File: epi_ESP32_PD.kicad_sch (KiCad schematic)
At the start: 53 parts, among them J1 Conn_01x08, J2 USB_C_Receptacle_USB2.0, J3 Conn_01x08, J4 Conn_01x02, J5 Conn_01x06, Q1 Q_PMOS_GDS, Q2 Q_NMOS_GDS, Q3 Q_NMOS_GDS, Q4 Q_NMOS_GDS, Q5 Q_NMOS_GDS, Q6 Q_NMOS_GDS, SW1 SW_MEC_5G, SW2 SW_MEC_5G, U1 ESP32-C3, U2 MIC5219-5.0YM5, U4 MIC5219-3.3YM5, Y1 Crystal

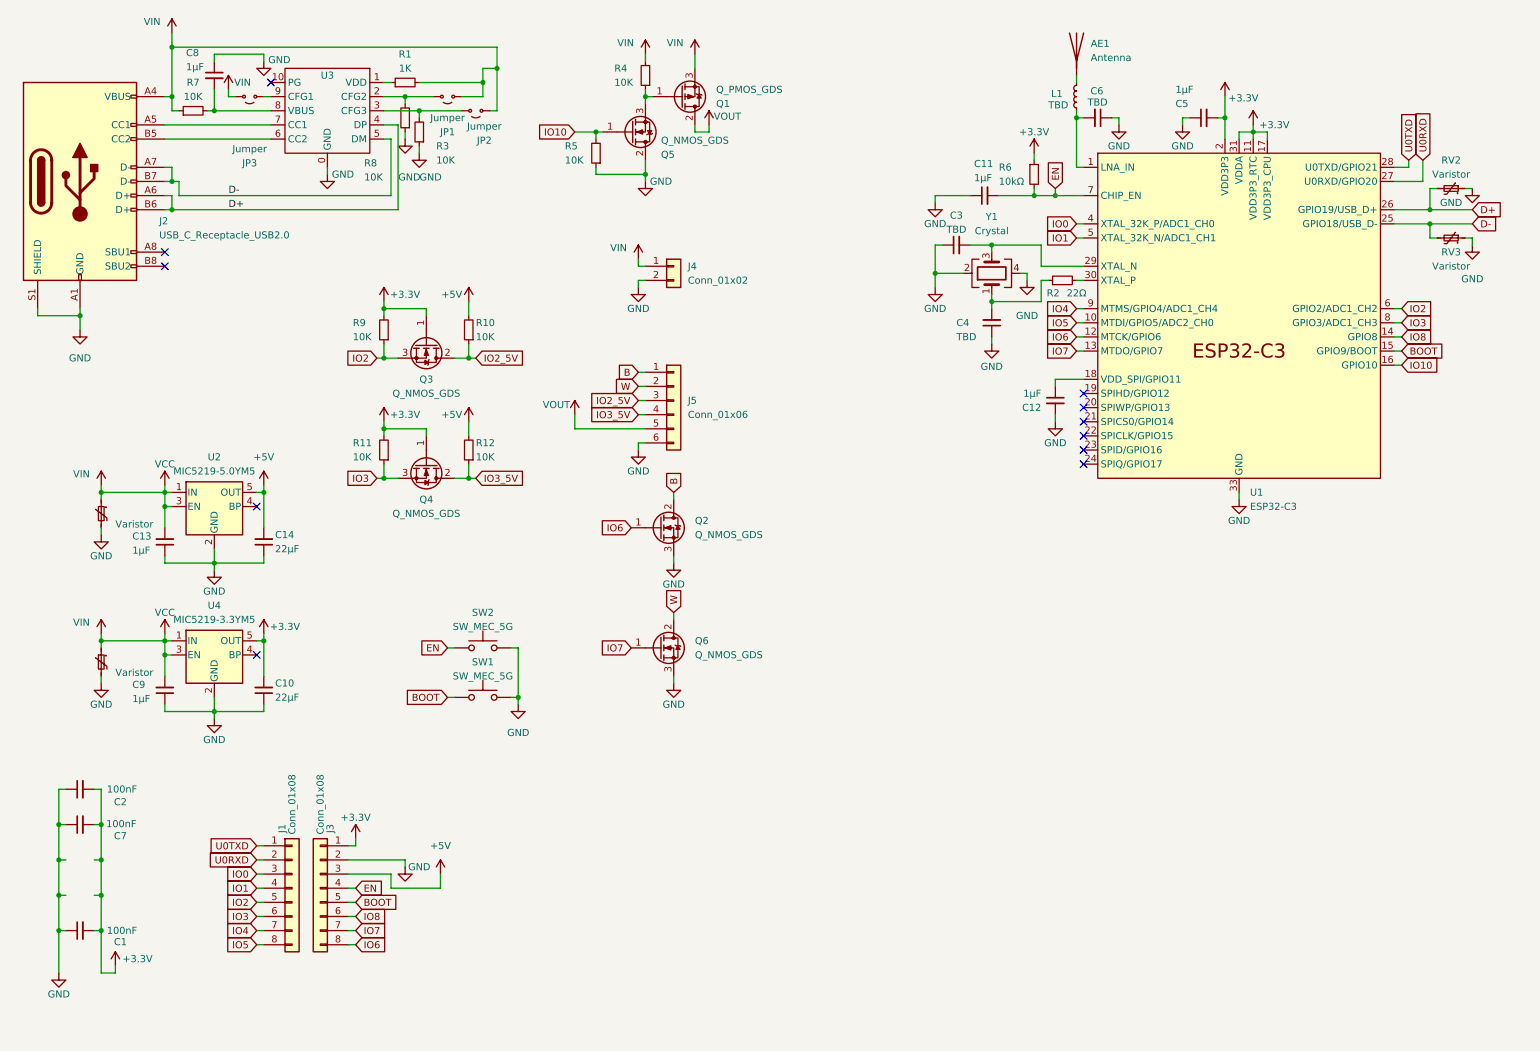
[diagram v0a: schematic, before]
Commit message: designed
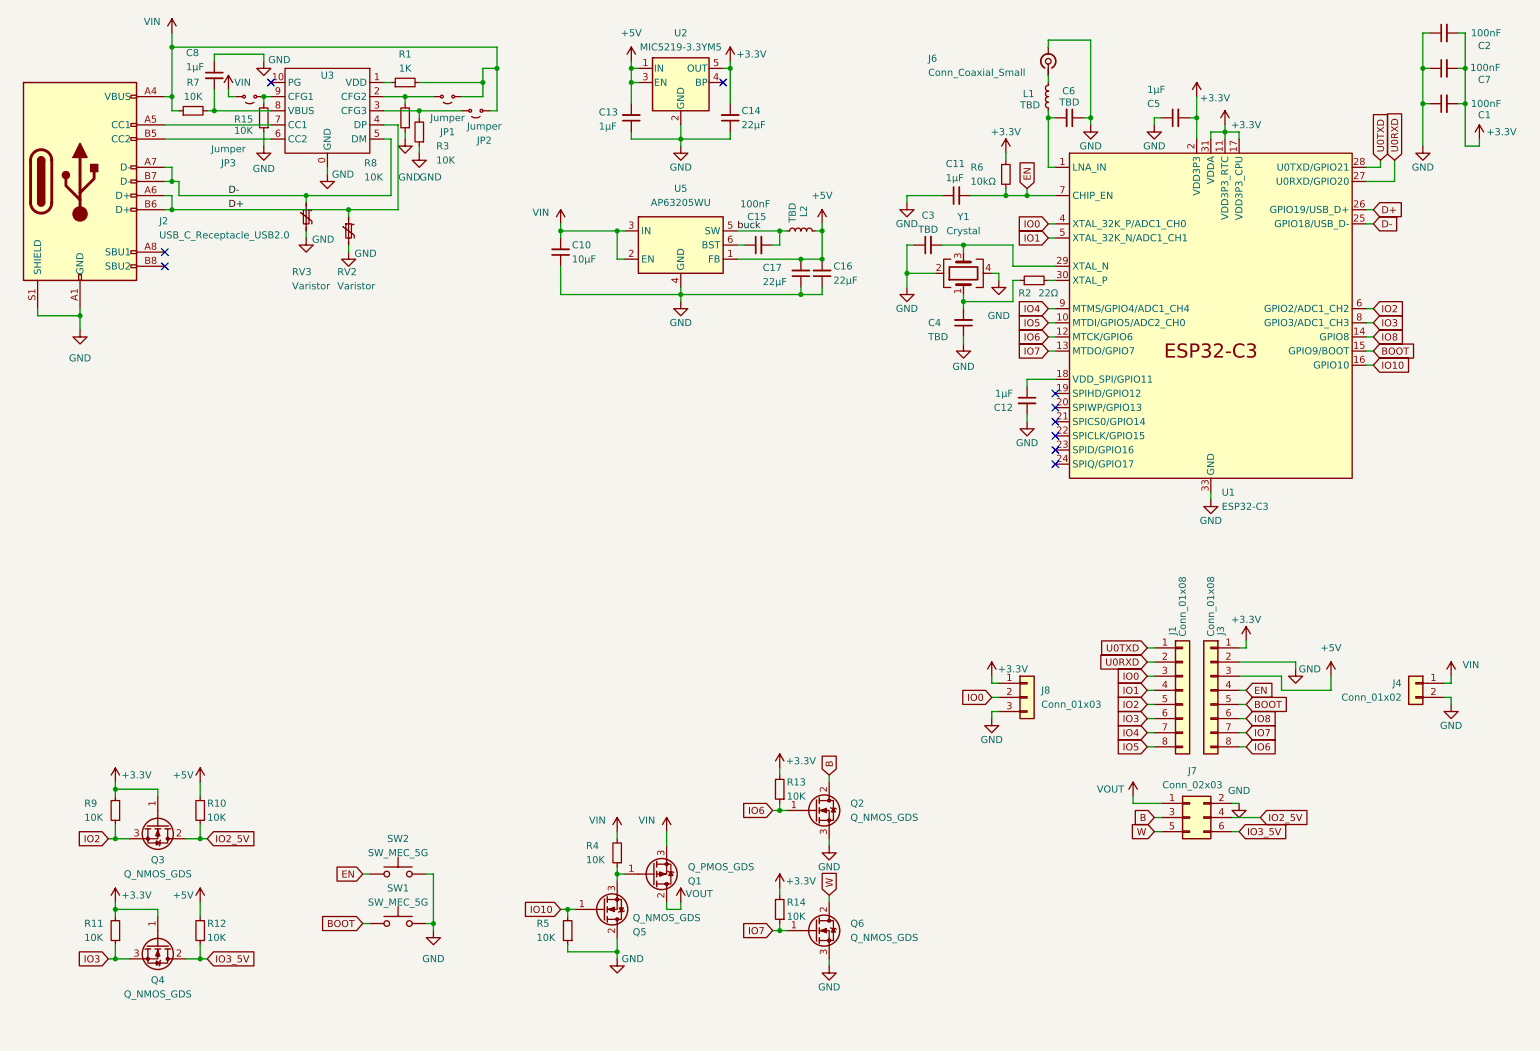
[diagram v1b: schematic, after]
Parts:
- removed AE1: Antenna, DIY:2450AT14A0100001T, symbol Device:Antenna
- removed C9: 1µF, Capacitor_SMD:C_0402_1005Metric, symbol Device:C_Small
- removed J5: Conn_01x06, Connector_PinHeader_1.27mm:PinHeader_1x06_P1.27mm_Horizontal, symbol Connector_Generic:Conn_01x06
- removed RV1, RV4: Varistor, Resistor_SMD:R_0402_1005Metric, symbol Device:Polyfuse_Small
- removed U4: MIC5219-3.3YM5, Package_TO_SOT_SMD:SOT-23-5, symbol Regulator_Linear:MIC5219-3.3YM5
- added C15: 100nF, Capacitor_SMD:C_0402_1005Metric, symbol Device:C_Small
- added C16, C17: 22µF, Capacitor_SMD:C_0805_2012Metric, symbol Device:C_Small
- added J6: Conn_Coaxial_Small, Connector_Coaxial:U.FL_Molex_MCRF_73412-0110_Vertical, symbol Connector:Conn_Coaxial_Small
- added J7: Conn_02x03, Connector_PinHeader_2.54mm:PinHeader_2x03_P2.54mm_Horizontal, symbol Connector_Generic:Conn_02x03_Odd_Even
- added J8: Conn_01x03, Connector_PinHeader_2.54mm:PinHeader_1x03_P2.54mm_Vertical, symbol Connector_Generic:Conn_01x03
- added L2: TBD, Inductor_SMD:L_Abracon_ASPI-0425, symbol Device:L_Small
- added R13, R14, R15: 10K, Resistor_SMD:R_0402_1005Metric, symbol Device:R_Small
- added U5: AP63205WU, Package_TO_SOT_SMD:TSOT-23-6, symbol Regulator_Switching:AP63203WU
- C10: value 22µF -> 10µF; footprint Capacitor_SMD:C_0603_1608Metric -> Capacitor_SMD:C_0805_2012Metric
- J1, J3: footprint Connector_PinHeader_1.27mm:PinHeader_1x08_P1.27mm_Vertical -> Connector_PinHeader_2.54mm:PinHeader_1x08_P2.54mm_Vertical
- U2: value MIC5219-5.0YM5 -> MIC5219-3.3YM5
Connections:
- net +3.3V: now also C14.2, U2.5 (OUT), J8.1 (Pin_1), R13.2, R14.2; no longer C10.2
- net +5V: now also C13.2, U2.1 (IN), U2.3 (EN), C16.2, C17.2, L2.2, U5.1 (FB); no longer C14.2, U2.5 (OUT)
- net B: now also J7.3 (Pin_3)
- net D+: now also RV2.1; no longer RV2.2
- net D-: now also RV3.1; no longer RV3.2
- net GND: now also RV2.2, RV3.2, C16.1, C17.1, J6.2 (Ext), J7.2 (Pin_2), J8.3 (Pin_3), R15.1, U5.4 (GND); no longer RV2.1, RV3.1
- net IO0: now also J8.2 (Pin_2)
- net IO2_5V: now also J7.4 (Pin_4)
- net IO3_5V: now also J7.6 (Pin_6)
- net IO6: now also R13.1
- net IO7: now also R14.1
- net VOUT: now also J7.1 (Pin_1)
- net W: now also J7.5 (Pin_5)
- net at JP3.1 (A), U3.9 (CFG1): now also R15.2
- net at L1.2: now also J6.1 (In)
- net VCC renamed VIN
- net VIN: now also C10.2, U5.2 (EN), U5.3 (IN); no longer C13.2, U2.1 (IN), U2.3 (EN)
- new net: C15.1, U5.6 (BST)
- new net buck: C15.2, L2.1, U5.5 (SW)
- no-connect marks 11 -> 10
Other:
- moved on the sheet: C1, C10, C11, C12, C13, C14, C2, C3, C4, C5, C6, C7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

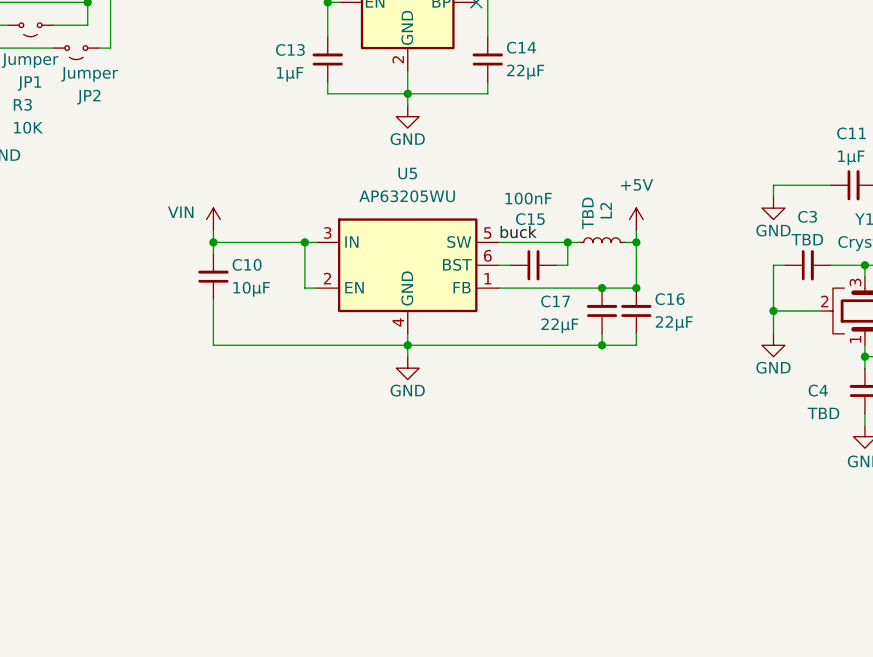
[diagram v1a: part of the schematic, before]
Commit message: made it pretty
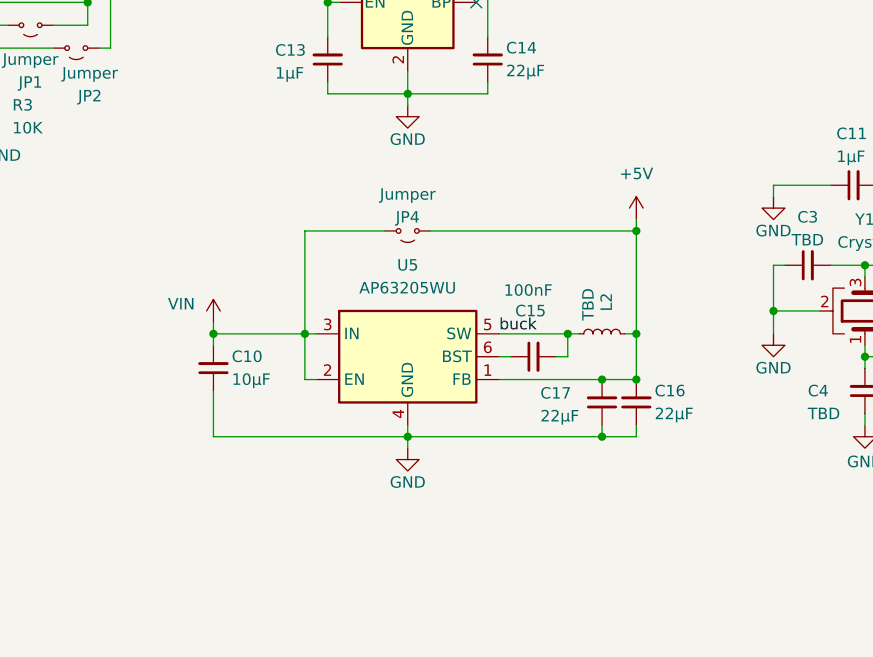
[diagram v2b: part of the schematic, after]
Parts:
- added JP4: Jumper, Jumper:SolderJumper-2_P1.3mm_Open_RoundedPad1.0x1.5mm, symbol Jumper:Jumper_2_Small_Open
- J2: footprint diy:USB-C MC-314C-4P16_V2 (2023_01_13 17_48_46 UTC) -> Connector_USB:USB_C_Receptacle_G-Switch_GT-USB-7010ASV
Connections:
- net +5V: now also JP4.1 (A)
- net VIN: now also JP4.2 (B)
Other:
- moved on the sheet: C10, C15, C16, C17, L2, U5

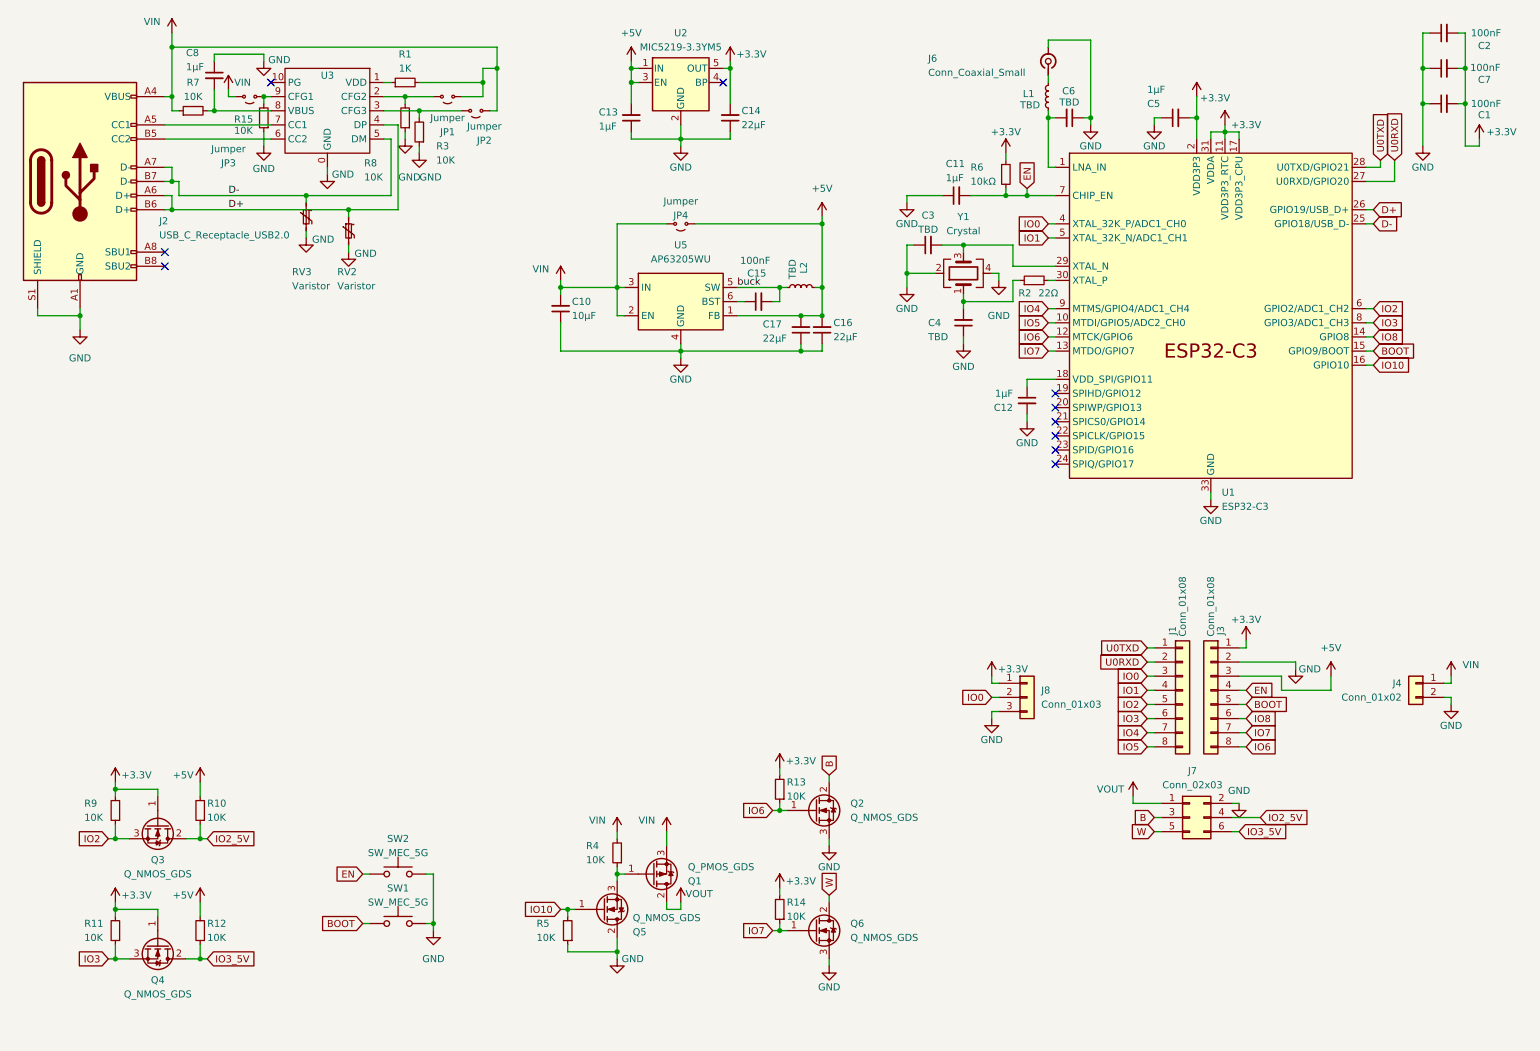
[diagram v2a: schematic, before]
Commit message: finishing touches
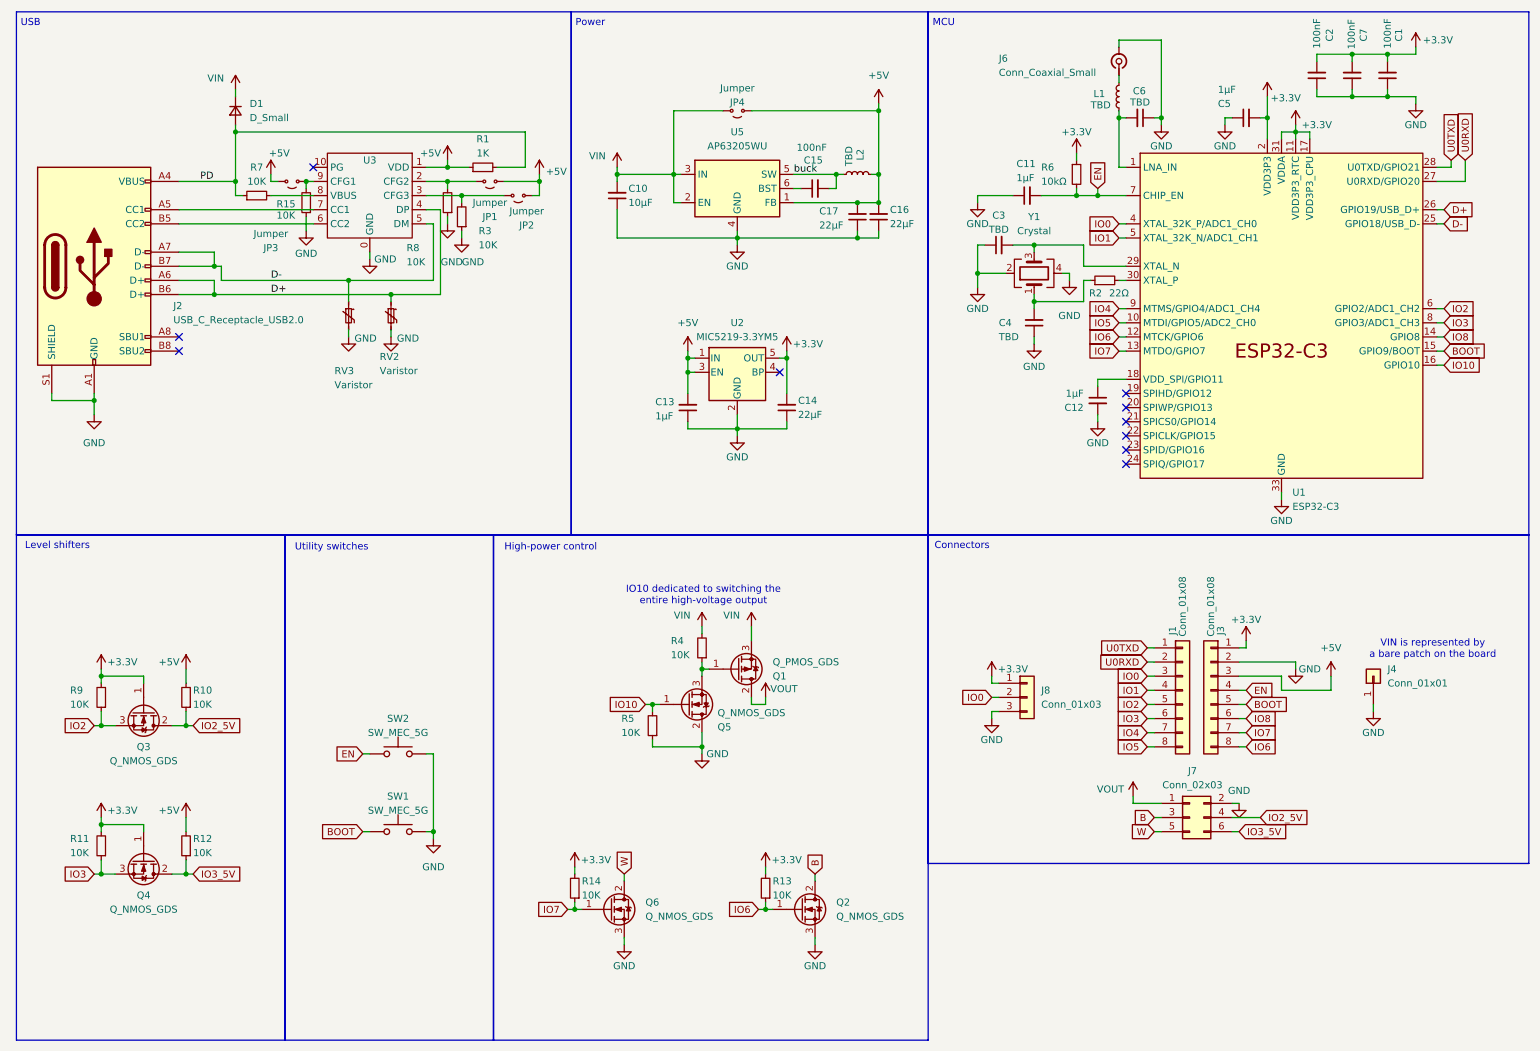
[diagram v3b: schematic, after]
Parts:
- removed C8: 1µF, Capacitor_SMD:C_0805_2012Metric, symbol Device:C_Small
- removed J4: Conn_01x02, Connector_PinHeader_2.54mm:PinHeader_1x02_P2.54mm_Vertical, symbol Connector_Generic:Conn_01x02
- added D1: D_Small, Diode_SMD:D_SOD-128, symbol Device:D_Small
- added J4: Conn_01x01, TestPoint:TestPoint_Pad_3.0x3.0mm, symbol Connector_Generic:Conn_01x01
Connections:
- net +5V: now also JP1.1 (A), JP2.1 (A), JP3.2 (B), R1.1, U3.1 (VDD)
- net GND: now also J4.1 (Pin_1)
- net VIN: now also D1.1 (K); no longer J2.A4 (VBUS), J2.A9 (VBUS), J2.B4 (VBUS), J2.B9 (VBUS), JP1.1 (A), JP2.1 (A), JP3.2 (B), R1.2, R7.1
- new net PD: D1.2 (A), J2.A4 (VBUS), J2.A9 (VBUS), J2.B4 (VBUS), J2.B9 (VBUS), R1.2, R7.1
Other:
- note added: "Connectors"
- note added: "High-power control"
- note added: "IO10 dedicated to switching the entire high-voltage output"
- note added: "Level shifters"
- note added: "MCU"
- note added: "Power"
- note added: "USB"
- note added: "Utility switches"
- note added: "VIN is represented by a bare patch on the board"
- moved on the sheet: C1, C10, C11, C12, C13, C14, C15, C16, C17, C2, C3, C4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
